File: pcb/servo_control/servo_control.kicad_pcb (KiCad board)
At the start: 2 copper layers, 94.6 x 66.7 mm, 80 parts, among them J1 Jack-DC, J10 Conn_01x03_Female, J11 Conn_01x03_Female, J12 Conn_01x03_Female, J13 Conn_01x03_Female, J14 Conn_01x03_Female, J15 Conn_01x03_Female, J16 Conn_01x03_Female, J17 Conn_01x03_Female, J18 Conn_01x03_Female, J19 Conn_01x03_Female, J2 YLIDAR X4, J20 Conn_01x03_Female, J21 Conn_01x06_Male, J22 GY-87, J3 Conn_01x03_Female, J4 Conn_01x03_Female, J5 Conn_01x03_Female, J6 Conn_01x03_Female, J7 Conn_01x03_Female, J8 Conn_01x03_Female, J9 Conn_01x03_Female, SW1 ESP_PROG, SW2 ESP_RST, U1 PCA9685PW, U2 LM317-3.3_SOT-223, U3 ESP32-WROOM-32, U4 MCP73213-A6SI/MF, U5 PCA9685PW, U6 LM317-5_SOT-223, U7 LT1085-ADJ

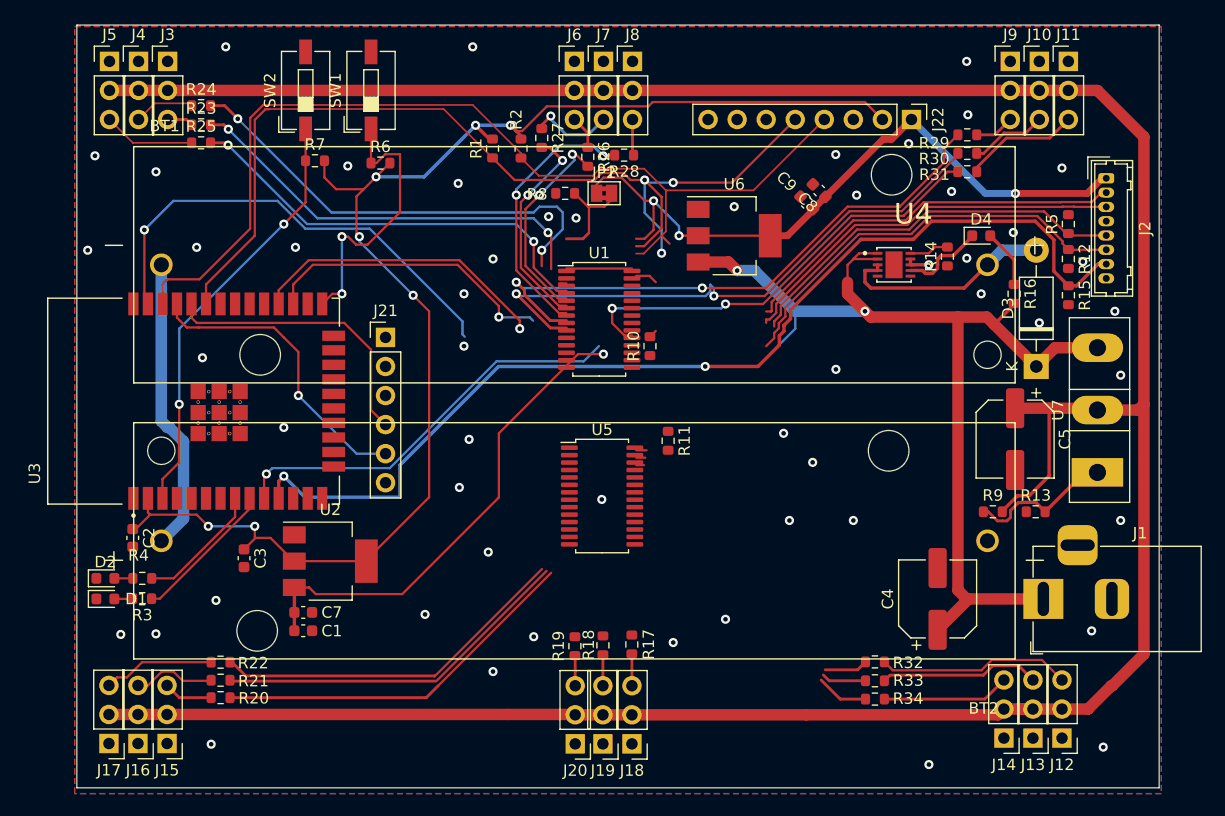
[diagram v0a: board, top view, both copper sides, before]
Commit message: move pcf
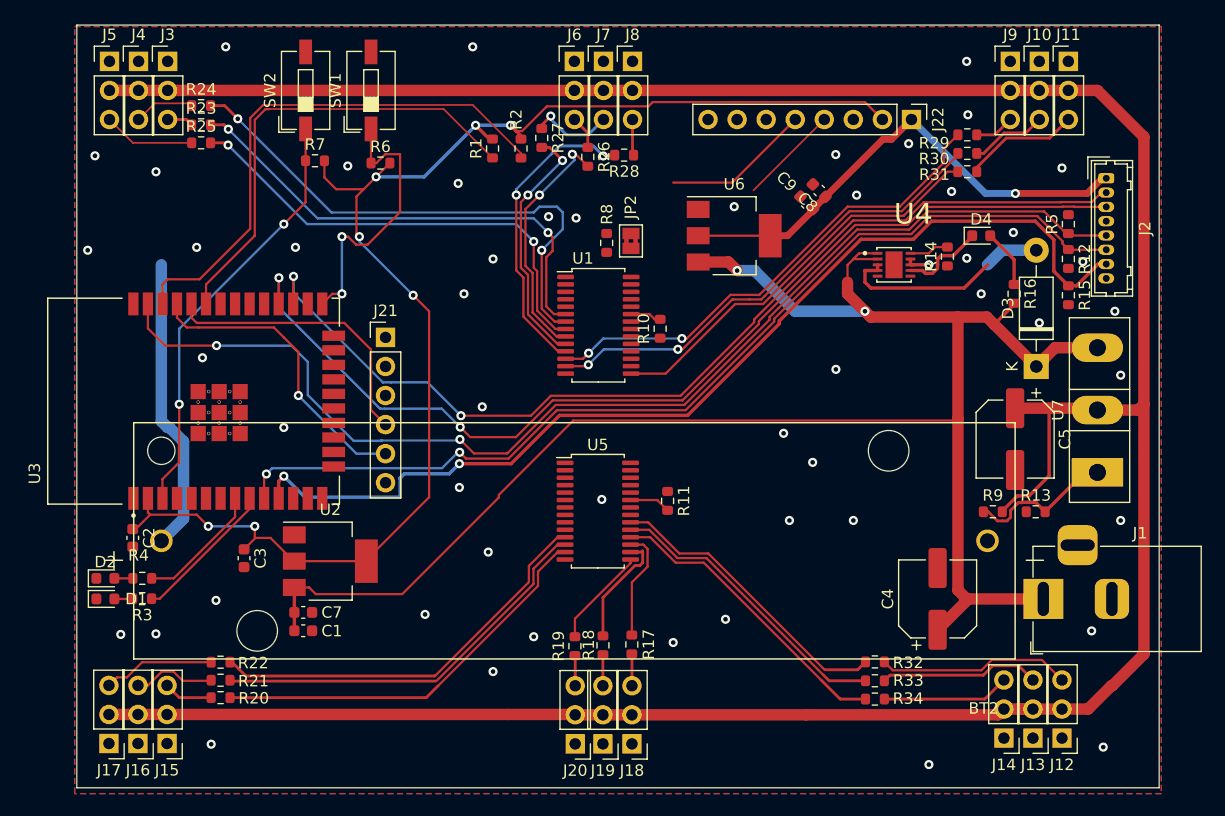
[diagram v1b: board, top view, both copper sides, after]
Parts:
- removed BT1: 1043, 18650:BAT_1043
- moved R8 5.65 mm to (147.6, 59.0), turned to 90 degrees
- moved R11 5.25 mm to (152.9, 81.6)
- moved JP2 4.78 mm to (149.7, 58.9), turned to 90 degrees
- moved R10 1.76 mm to (152.3, 66.5)
- moved U5 1.38 mm to (146.8, 82.5)
- moved U1 0.53 mm to (146.9, 66.2)
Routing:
- net I2C_SDA: track 89.5 -> 54.1 mm, vias 3 -> 0
- net I2C_SCL: track 86.8 -> 56.1 mm
- net ESP_TX: track 60.8 -> 90.4 mm, vias 1 -> 2
- net ESP_RX: track 60.5 -> 87.6 mm, vias 1 -> 2
- net M_SCTR: track 76.0 -> 102.5 mm, vias 1 -> 2
- net PWM_1_13: track 3.81 -> 26.2 mm
- net PWM_1_12: track 3.90 -> 26.0 mm
- net PWM_1_11: track 4.57 -> 26.4 mm
- net 9V: track 135.8 -> 156.6 mm, vias 3 -> 2
- net 5V: track 61.1 -> 43.3 mm, vias 3 -> 1
- net DEV_EN: track 72.7 -> 86.9 mm, vias 1 -> 2
- net PWM_1_9: track 0.02 -> 10.2 mm
- net PWM_1_10: track 0.00 -> 9.74 mm
- net PWM_0_7: track 51.1 -> 42.1 mm
- net FIRST_A0: track 8.99 -> 0.00 mm
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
